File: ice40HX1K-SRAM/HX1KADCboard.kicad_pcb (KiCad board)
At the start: 4 copper layers, 141.9 x 92.2 mm, 142 parts, among them J1 Conn_01x03_Male, J2 Conn_02x05_Odd_Even, J3 Conn_01x20_Male, J5 Conn_01x06_Male, J6 Conn_01x05, U1 LTC3406ES5, U10 FAN5341, U11 FAN5341, U12 FAN5341, U13 FAN5341, U2 MAX40200AUK, U3 LTC3406ES5, U4 MAX40200AUK, U5 AT25SF081-SSHD-X, U6 ICE40HX1K-VQ100(VQFP100), U7 AS7C34096A, U8 ATSAMD11D14A-SS, U9 BL652, X1 USBFCI_10103594_MILL, X2 ASE-10MHz, X3 ASE-10MHz, X4 ASE-10MHz, X5 ASV-xxxMHz, X6 ASV-xxxMHz, X7 ASV-xxxMHz

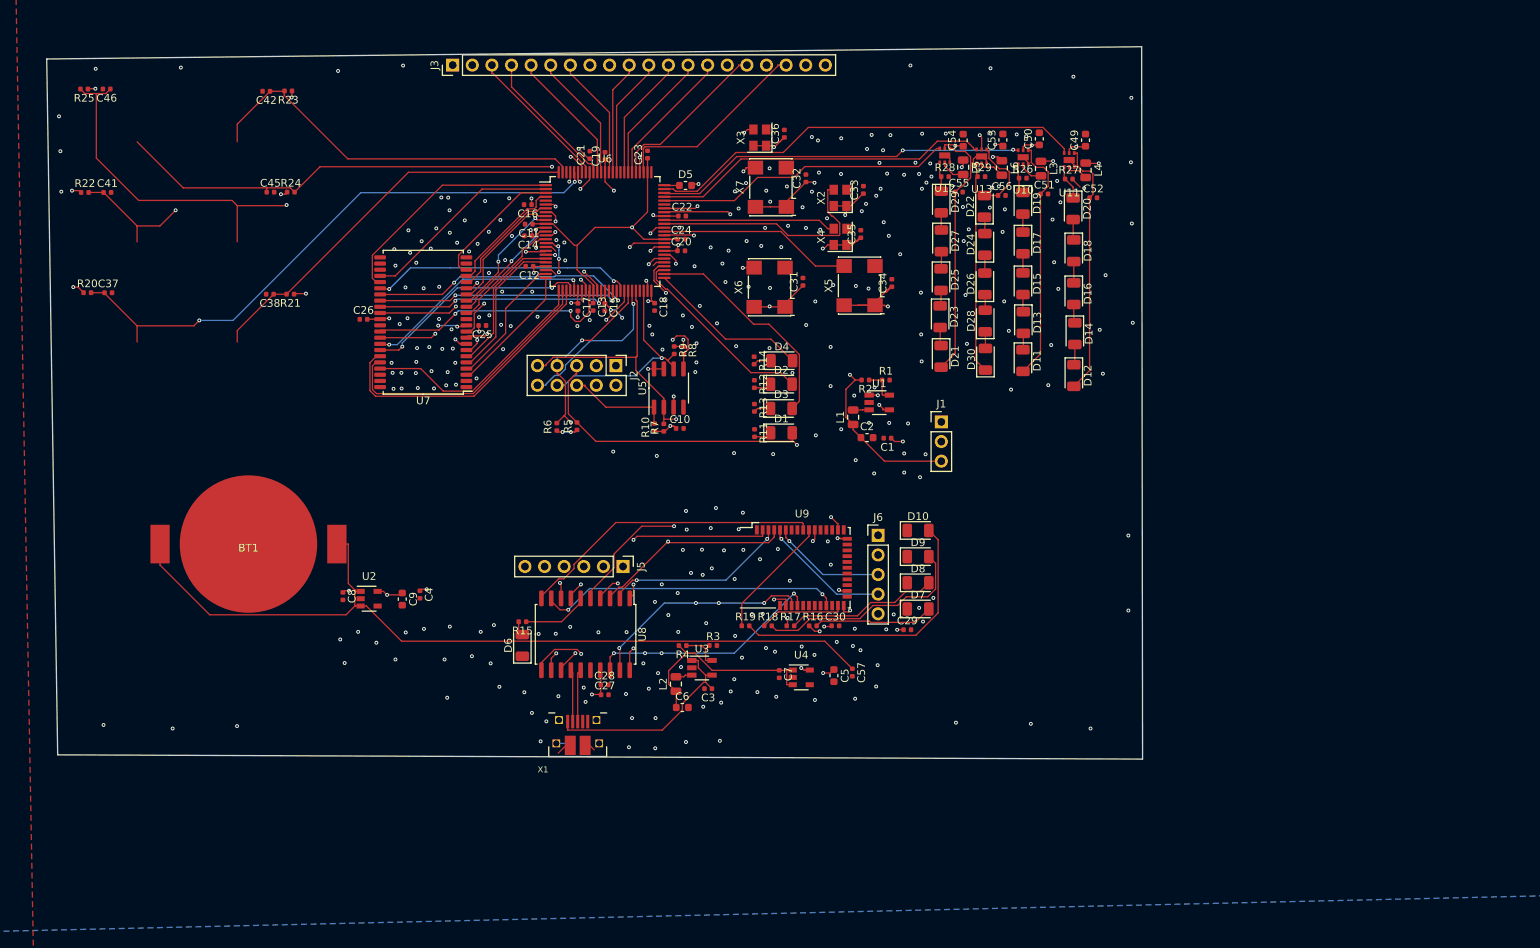
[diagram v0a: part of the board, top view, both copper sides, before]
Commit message: fpgaNext-2
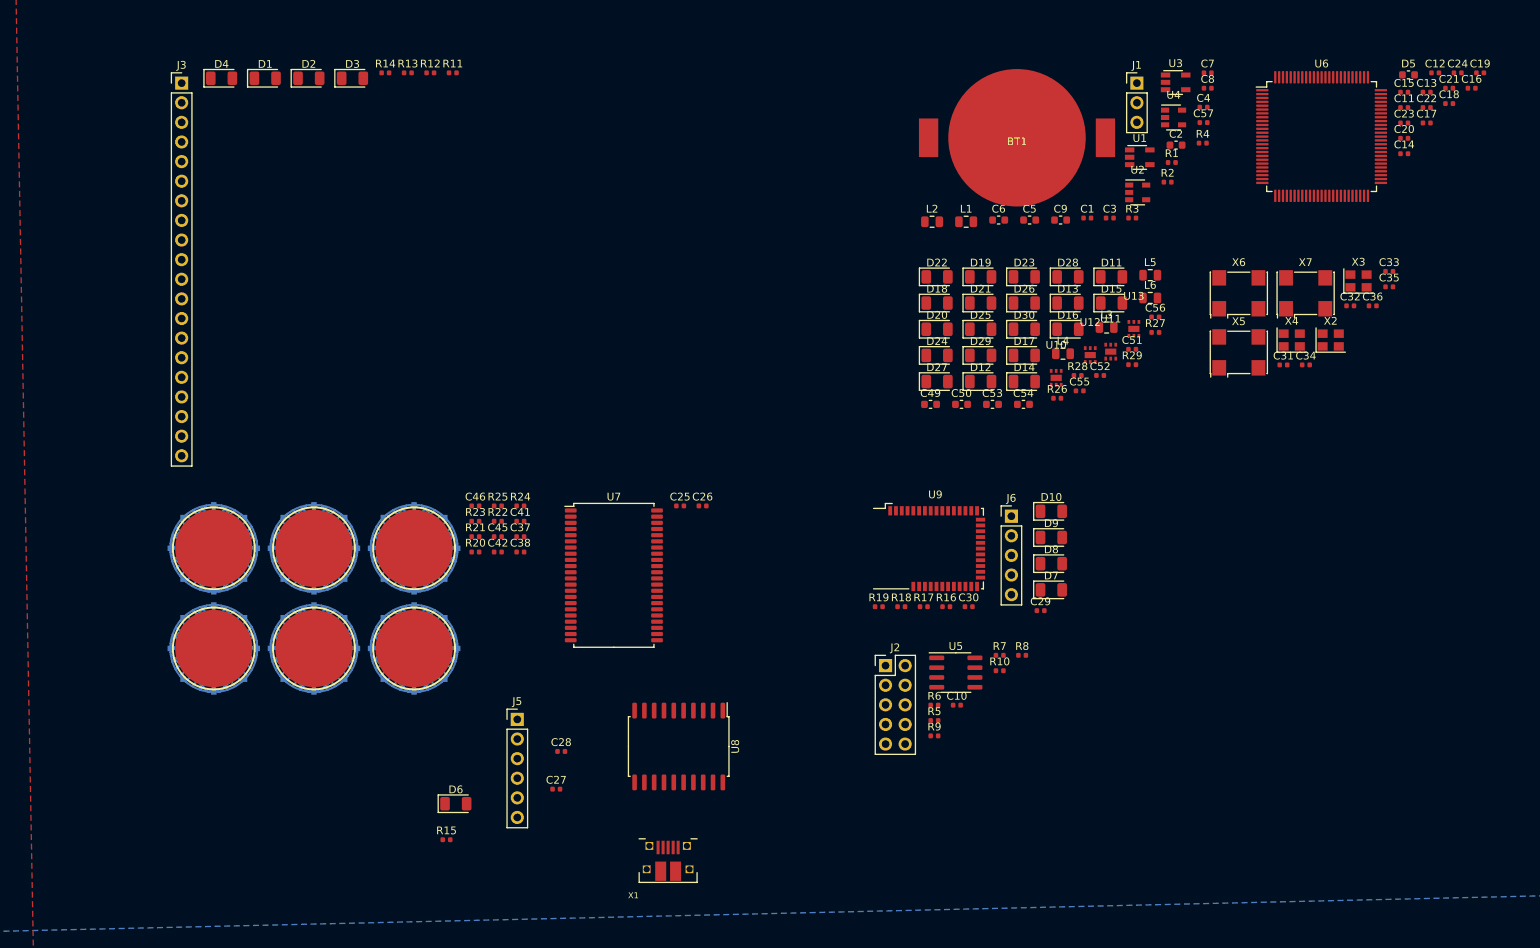
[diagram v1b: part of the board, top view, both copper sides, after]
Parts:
- added C39: Ccap, kifootp:CAPBUTTON, F.Cu at (80.4, 105.2)
- added C40: Ccap, kifootp:CAPBUTTON, F.Cu at (80.4, 118.2)
- added C43: Ccap, kifootp:CAPBUTTON, F.Cu at (93.4, 105.2)
- added C44: Ccap, kifootp:CAPBUTTON, F.Cu at (106.4, 118.2)
- added C47: Ccap, kifootp:CAPBUTTON, F.Cu at (106.4, 105.2)
- added C48: Ccap, kifootp:CAPBUTTON, F.Cu at (93.4, 118.2)
- moved C8 129.9 mm to (209.1, 45.6), turned to 0 degrees
- moved C16 123.2 mm to (243.3, 45.6), turned to 0 degrees
- moved C12 119.9 mm to (238.6, 43.6), turned to 0 degrees
- moved C4 119.5 mm to (208.6, 48.1), turned to 0 degrees
- moved C11 114.4 mm to (234.6, 48.1), turned to 0 degrees
- moved C14 113.9 mm to (234.6, 54.1), turned to 0 degrees
- moved C19 113.8 mm to (244.4, 43.6), turned to 0 degrees
- moved U2 112.6 mm to (200.1, 59.1)
- moved BT1 112.6 mm to (184.4, 52.0)
- moved C17 112.5 mm to (237.5, 50.1), turned to 0 degrees
- moved C21 111.6 mm to (240.4, 45.6), turned to 0 degrees
- moved C13 111.5 mm to (237.5, 46.1), turned to 0 degrees
- moved C15 107.2 mm to (234.6, 46.1), turned to 0 degrees
- moved C18 106.2 mm to (240.4, 47.6), turned to 0 degrees
- moved C24 102.8 mm to (241.5, 43.6)
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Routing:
- net +3V3: track 142.8 -> 0.00 mm, vias 58 -> 0
- net Net-(BT1-Pad1): track 109.5 -> 0.00 mm
- net CDONE: track 102.2 -> 0.00 mm, vias 6 -> 0
- net +1V2: track 98.1 -> 0.00 mm, vias 3 -> 0
- net SPI_SCK: track 87.3 -> 0.00 mm, vias 4 -> 0
- net SPI_OUT: track 86.7 -> 0.00 mm, vias 3 -> 0
- net CRESET: track 85.3 -> 0.00 mm, vias 6 -> 0
- net IO97: track 83.8 -> 0.00 mm, vias 2 -> 0
- net SPI_CS: track 80.8 -> 0.00 mm, vias 3 -> 0
- net SPI_IN: track 78.0 -> 0.00 mm, vias 3 -> 0
- net IO96: track 75.6 -> 0.00 mm, vias 2 -> 0
- net IO95: track 71.2 -> 0.00 mm, vias 3 -> 0
- net IO94: track 64.0 -> 0.00 mm, vias 2 -> 0
- net IO74: track 57.0 -> 0.00 mm
- net IO64: track 56.3 -> 0.00 mm, vias 2 -> 0
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- removed copper zone on In2.Cu, net +3V3
- removed copper zone on In1.Cu, net GND
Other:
- board outline removed
- copper layers 4 -> 2
